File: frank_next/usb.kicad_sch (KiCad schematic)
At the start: 44 parts, among them J10 USB4215-03-A, J11 USB4215-03-A, J8 676430910, J9 676430910, U10 TPD4S012DRYR, U11 TPD4S012DRYR, U12 TPD4S012DRYR, U13 TPS2116DRL, U14 TS3USB221RSER, U15 AMS1117-3.3, U16 CH334F, U9 TPD4S012DRYR, Y3 12MHz

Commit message: Board updates
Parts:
- S6: footprint FRANK:SK12D07VG3NS_PWR -> FRANK:Switch_Slide_SK12D07VG3NS_PWR
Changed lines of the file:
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@@
 			)
 		)
-		(property "Footprint" "FRANK:SK12D07VG3NS_PWR"
+		(property "Footprint" "FRANK:Switch_Slide_SK12D07VG3NS_PWR"
 			(at 134.62 -55.55 0)
 			(hide yes)

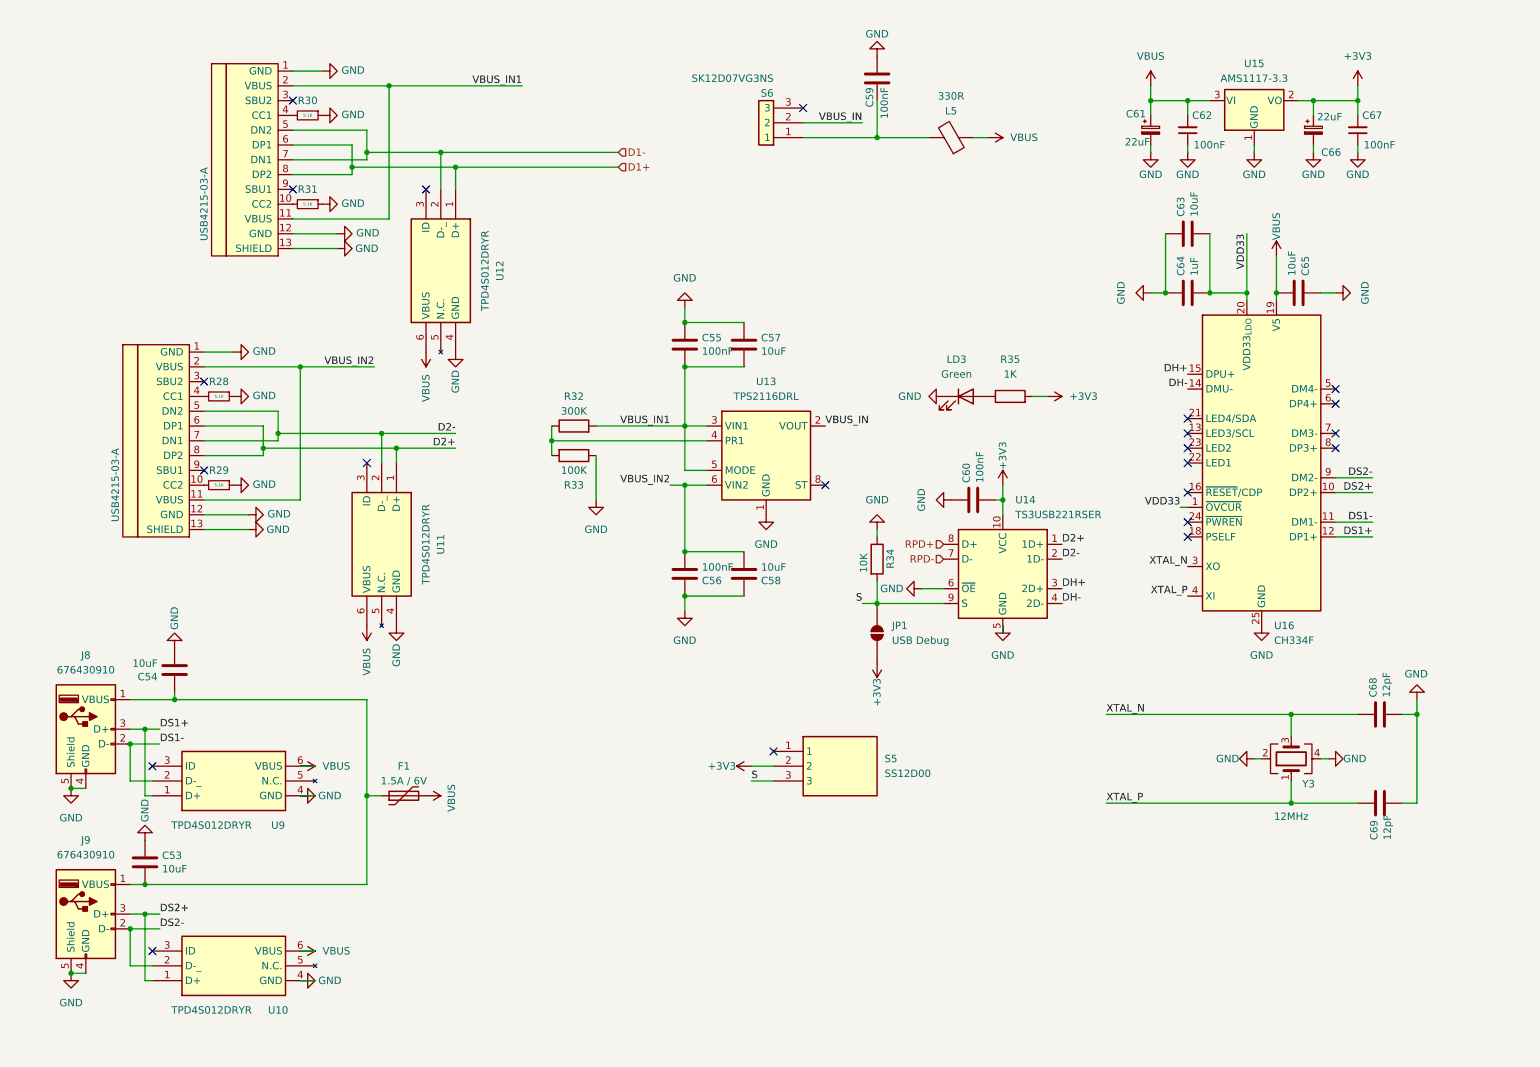
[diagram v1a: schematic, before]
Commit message: FRANK Next updates
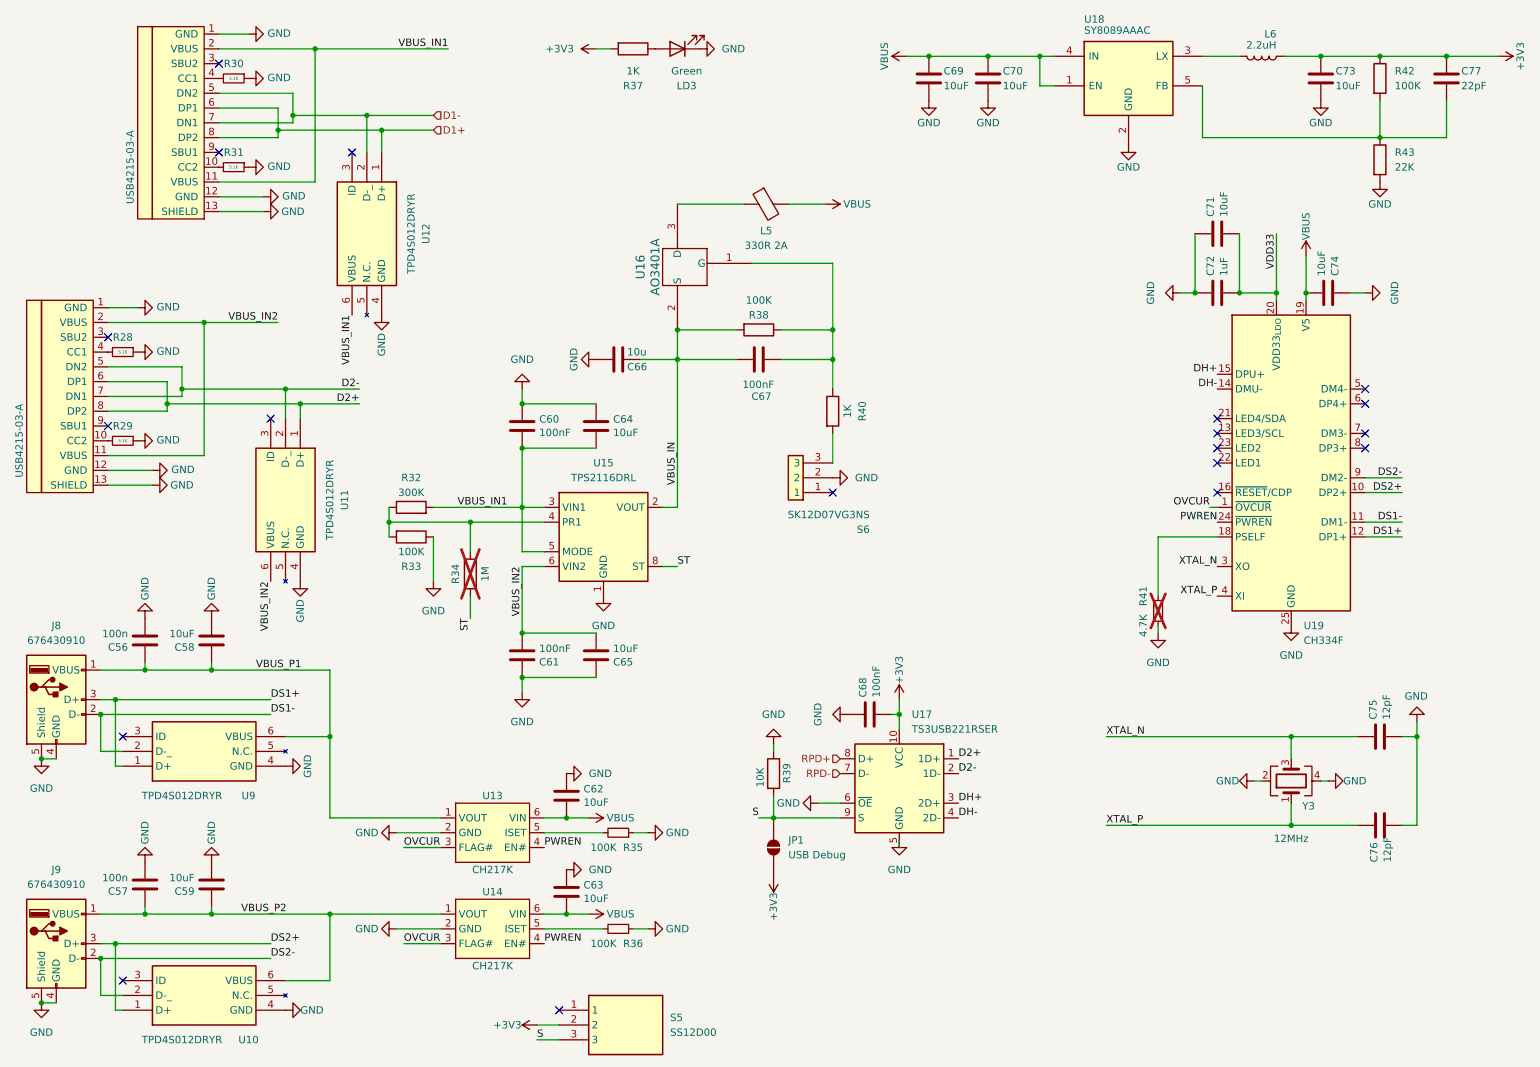
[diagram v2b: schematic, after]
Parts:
- removed C53: 10uF, FRANK:C_0603_1608Metric, symbol FRANK:C
- removed C61, C66: 22uF, FRANK:CP_Tantalum_3528-12, symbol FRANK:C_Polarized_Small
- removed C62, C67: 100nF, FRANK:C_0603_1608Metric, symbol FRANK:C_Small
- removed F1: 1.5A / 6V, FRANK:Fuse_1206_3216Metric, symbol FRANK:Polyfuse
- removed J9: 676430910, FRANK:USB_A_Short, symbol FRANK:USB_A
- removed U10: TPD4S012DRYR, FRANK:TPD4S012DRYR, symbol FRANK:TPD4S012DRYR
- removed U15: AMS1117-3.3, FRANK:SOT-89-3, symbol FRANK:AMS1117-3.3
- added C56: 100n, FRANK:C_0603_1608Metric, symbol FRANK:C
- added C58, C59, C62, C63, C69, C70, C73: 10uF, FRANK:C_0603_1608Metric, symbol FRANK:C
- added C67: 100nF, FRANK:C_0603_1608Metric, symbol FRANK:C
- added C77: 22pF, FRANK:C_0603_1608Metric, symbol FRANK:C
- added J8: 676430910, FRANK:USB_A_Short, symbol FRANK:USB_A
- added L6: 2.2uH, Inductor_SMD:L_Cenker_CKCS3015, symbol FRANK:L
- added R34: 1M, FRANK:R_0603_1608Metric, symbol FRANK:R
- added R35, R36: 100K, FRANK:R_0603_1608Metric, symbol Device:R_Small
- added R38, R42: 100K, FRANK:R_0603_1608Metric, symbol FRANK:R
- added R40: 1K, FRANK:R_0603_1608Metric, symbol FRANK:R
- added R41: 4.7K, FRANK:R_0603_1608Metric, symbol Device:R_Small
- added R43: 22K, FRANK:R_0603_1608Metric, symbol FRANK:R
- added U13, U14: CH217K, Package_TO_SOT_SMD:SOT-23-6, symbol FRANK:CH217K
- added U16: AO3401A, FRANK:SOT-23-3L_AOS, symbol FRANK:AO3401A
- added U18: SY8089AAAC, Package_TO_SOT_SMD:SOT-23-5, symbol FRANK:SY8089AAAC
- added U9: TPD4S012DRYR, FRANK:TPD4S012DRYR, symbol FRANK:TPD4S012DRYR
- C57: renamed from C54; value 10uF -> 100n
- C66: renamed from C59; value 100nF -> 10u
- L5: value 330R -> 330R 2A; footprint FRANK:L_0603_1608Metric -> Inductor_SMD:L_0805_2012Metric
- Y3: footprint FRANK:Crystal_SMD_2520-4Pin_2.5x2.0mm -> FRANK:Crystal_SMD_3225-4Pin_3.2x2.5mm
- renumbered C55 to C60, C56 to C61, C57 to C64, C58 to C65, C60 to C68, C63 to C71, C64 to C72, C65 to C74, C68 to C75, C69 to C76, J8 to J9, R35 to R37, R34 to R39, U9 to U10, U13 to U15, U14 to U17, U16 to U19
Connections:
- net +3V3: now also C73.1, C77.1, L6.1, R42.1
- net DS1+: now also J8.3 (D+), U9.1 (D+); no longer J9.3 (D+), U10.1 (D+)
- net DS1-: now also J8.2 (D-), U9.2 (D-_); no longer J9.2 (D-), U10.2 (D-_)
- net DS2+: now also J9.3 (D+), U10.1 (D+)
- net DS2-: now also J9.2 (D-), U10.2 (D-_)
- net GND: now also S6.2, C56.2, C58.2, C59.2, C62.1, C63.1, C69.2, C70.2, C73.2, J8.4 (GND), J8.5 (Shield), R35.1, R36.1, R41.2, R43.2, U13.2 (GND), U14.2 (GND), U18.2 (GND), U9.4 (GND)
- net VBUS: now also L5.2, C62.2, C63.2, C69.1, C70.1, U13.6 (VIN), U14.6 (VIN), U18.1 (EN), U18.4 (IN); no longer L5.1, U10.6 (VBUS), U11.6 (VBUS), U12.6 (VBUS)
- net VBUS_IN: now also C66.1, C67.2, R38.2, U16.2 (S); no longer S6.2
- net VBUS_IN1: now also U12.6 (VBUS)
- net VBUS_IN2: now also U11.6 (VBUS)
- net VDD33: no longer U19.1 (~{OVCUR})
- net at S6.3: now also R40.2
- net at R32.1, R33.2, U15.4 (PR1): now also R34.1
- net VBUS_P2: now reaches C57.1, J9.1 (VBUS)
- net VBUS_P2: now also U10.6 (VBUS), C59.1, U14.1 (VOUT)
- net ST: now reaches U15.8 (ST)
- net ST: now also R34.2
- net at U19.18 (PSELF): now also R41.1
- net PWREN: now reaches U19.24 (~{PWREN})
- net PWREN: now also U13.4 (EN#), U14.4 (EN#)
- new net: R36.2, U14.5 (ISET)
- new net: C67.1, R38.1, R40.1, U16.1 (G)
- new net: L6.2, U18.3 (LX)
- new net: C77.2, R42.2, R43.1, U18.5 (FB)
- new net: R35.2, U13.5 (ISET)
- new net: L5.1, U16.3 (D)
- new net OVCUR: U13.3 (FLAG#), U14.3 (FLAG#), U19.1 (~{OVCUR})
- new net VBUS_P1: C56.1, C58.1, J8.1 (VBUS), U13.1 (VOUT), U9.6 (VBUS)
- now unconnected: S6.1
- no-connect marks 22 -> 19
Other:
- moved on the sheet: C57, C60, C61, C64, C65, C66, C68, C71, C72, C74, C75, C76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

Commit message: FRANK Next WIP
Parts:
- L6: footprint Inductor_SMD:L_Cenker_CKCS3015 -> FRANK:L_Cenker_CKCS3015
- U18: footprint Package_TO_SOT_SMD:SOT-23-5 -> FRANK:SOT-23-5
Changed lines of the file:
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@@
 			)
 		)
-		(property "Footprint" "Inductor_SMD:L_Cenker_CKCS3015"
+		(property "Footprint" "FRANK:L_Cenker_CKCS3015"
 			(at 232.41 22.86 0)
 			(hide yes)
@@
 			)
 		)
-		(property "Footprint" "Package_TO_SOT_SMD:SOT-23-5"
+		(property "Footprint" "FRANK:SOT-23-5"
 			(at 209.55 25.4 0)
 			(hide yes)

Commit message: FRANK Next 1.01 WIP
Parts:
- L5: footprint Inductor_SMD:L_0805_2012Metric -> FRANK:L_0805_2012Metric
- R35, R36, R41: symbol Device:R_Small -> FRANK:R_Small
- U13, U14: footprint Package_TO_SOT_SMD:SOT-23-6 -> FRANK:SOT-23-6
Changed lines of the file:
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@@
 			)
 		)
-		(property "Footprint" "Package_TO_SOT_SMD:SOT-23-6"
+		(property "Footprint" "FRANK:SOT-23-6"
 			(at 93.98 177.8 0)
 			(hide yes)
@@
 	(symbol
 		(lib_name "R_Small_4")
-		(lib_id "Device:R_Small")
+		(lib_id "FRANK:R_Small")
 		(at 121.92 172.72 270)
 		(mirror x)
@@
 	)
 	(symbol
-		(lib_id "Device:R_Small")
+		(lib_id "FRANK:R_Small")
 		(at 214.63 118.11 0)
 		(unit 1)
@@
 	(symbol
 		(lib_name "R_Small_1")
-		(lib_id "Device:R_Small")
+		(lib_id "FRANK:R_Small")
 		(at 121.92 156.21 270)
 		(mirror x)
@@
 			)
 		)
-		(property "Footprint" "Inductor_SMD:L_0805_2012Metric"
+		(property "Footprint" "FRANK:L_0805_2012Metric"
 			(at 147.32 46.482 90)
 			(hide yes)
@@
 			)
 		)
-		(property "Footprint" "Package_TO_SOT_SMD:SOT-23-6"
+		(property "Footprint" "FRANK:SOT-23-6"
 			(at 93.98 161.29 0)
 			(hide yes)
